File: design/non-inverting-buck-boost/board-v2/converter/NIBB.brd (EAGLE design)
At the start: 64.7 x 43.2 mm, 10 parts

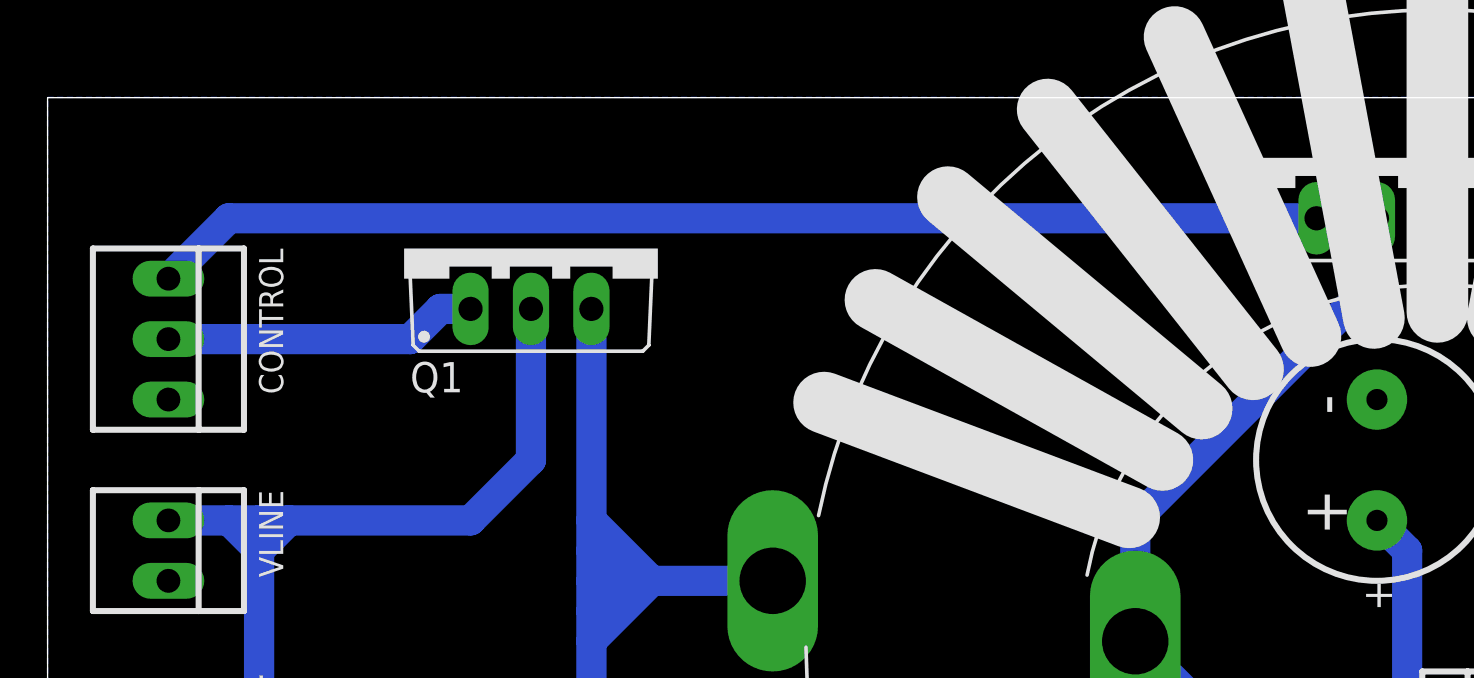
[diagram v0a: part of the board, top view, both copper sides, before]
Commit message: updated mosfet conections
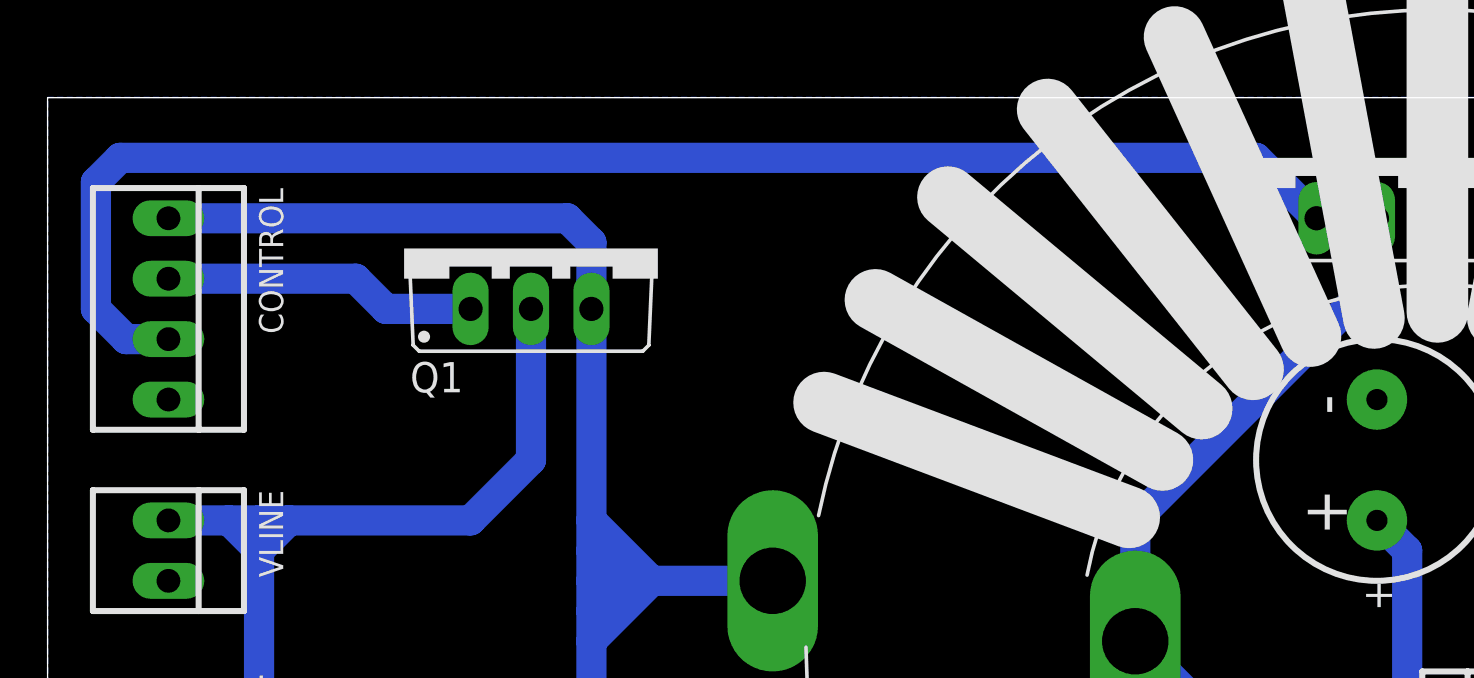
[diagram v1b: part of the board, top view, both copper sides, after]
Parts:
- CONTROL: value 22-23-2031 -> 22-23-2041; device con-molex:22-23-2031 -> con-molex:22-23-2041
- moved CONTROL 1.27 mm to (5.08, 34.3)
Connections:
- net CONTROL2 renamed N$4
- removed net CONTROL1: CONTROL.1, Q2.G
- new net N$5: CONTROL.3, Q2.G
- net GND: now also CONTROL.4; no longer CONTROL.3
- net N$1: now also CONTROL.1
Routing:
- net N$5: track 0.00 -> 61.7 mm
- net CONTROL1: track 49.3 -> 0.00 mm
- net N$1: track 42.5 -> 63.5 mm
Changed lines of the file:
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@@
 <element name="Q1" library="felippe" package="TO220BV" value="" x="20.32" y="36.83"/>
 <element name="Q2" library="felippe" package="TO220BV" value="" x="55.88" y="40.64"/>
-<element name="CONTROL" library="con-molex" package="22-23-2031" value="22-23-2031" x="5.08" y="33.02" rot="R270">
-<attribute name="MF" value="MOLEX" x="5.08" y="33.02" size="1.778" layer="27" rot="R270" display="off"/>
-<attribute name="MPN" value="22-23-2031" x="5.08" y="33.02" size="1.778" layer="27" rot="R270" display="off"/>
-<attribute name="OC_FARNELL" value="1462950" x="5.08" y="33.02" size="1.778" layer="27" rot="R270" display="off"/>
-<attribute name="OC_NEWARK" value="30C0862" x="5.08" y="33.02" size="1.778" layer="27" rot="R270" display="off"/>
-</element>
 <element name="CIN" library="capacitor" package="20ROUND40P" value="" x="8.89" y="12.7" rot="R270">
 <attribute name="DESC" value="Capacitor, polarized" x="8.89" y="12.7" size="1.778" layer="27" rot="R270" display="off"/>
+</element>
+<element name="CONTROL" library="con-molex" package="22-23-2041" value="22-23-2041" x="5.08" y="34.29" rot="R270">
+<attribute name="MF" value="MOLEX" x="5.08" y="34.29" size="1.778" layer="27" rot="R270" display="off"/>
+<attribute name="MPN" value="22-23-2041" x="5.08" y="34.29" size="1.778" layer="27" rot="R270" display="off"/>
+<attribute name="OC_FARNELL" value="1462920" x="5.08" y="34.29" size="1.778" layer="27" rot="R270" display="off"/>
+<attribute name="OC_NEWARK" value="38C0355" x="5.08" y="34.29" size="1.778" layer="27" rot="R270" display="off"/>
 </element>
 </elements>
@@
 <wire x1="20.32" y1="27.94" x2="20.32" y2="34.29" width="1.27" layer="16"/>
 </signal>
-<signal name="CONTROL1">
-<contactref element="Q2" pad="G"/>
-<contactref element="CONTROL" pad="1"/>
-<wire x1="5.08" y1="35.56" x2="7.62" y2="38.1" width="1.27" layer="16"/>
-<wire x1="7.62" y1="38.1" x2="53.34" y2="38.1" width="1.27" layer="16"/>
-</signal>
 <signal name="N$7">
 <contactref element="D2" pad="C"/>
@@
 <wire x1="22.86" y1="24.13" x2="22.86" y2="22.86" width="1.27" layer="16"/>
 <wire x1="22.86" y1="24.13" x2="22.86" y2="25.4" width="1.27" layer="16"/>
-<wire x1="22.86" y1="25.4" x2="22.86" y2="34.29" width="1.27" layer="16"/>
+<wire x1="22.86" y1="34.29" x2="22.86" y2="25.4" width="1.27" layer="16"/>
 <wire x1="22.86" y1="22.86" x2="22.86" y2="21.59" width="1.27" layer="16"/>
 <wire x1="22.86" y1="21.59" x2="22.86" y2="20.32" width="1.27" layer="16"/>
@@
 <wire x1="22.86" y1="21.59" x2="24.13" y2="22.86" width="1.27" layer="16"/>
 <wire x1="24.13" y1="22.86" x2="22.86" y2="24.13" width="1.27" layer="16"/>
+<contactref element="CONTROL" pad="1"/>
+<wire x1="5.08" y1="38.1" x2="21.844" y2="38.1" width="1.27" layer="16"/>
+<wire x1="21.844" y1="38.1" x2="22.86" y2="37.084" width="1.27" layer="16"/>
+<wire x1="22.86" y1="37.084" x2="22.86" y2="34.29" width="1.27" layer="16"/>
 </signal>
 <signal name="GND">
@@
 <contactref element="OUT" pad="2"/>
 <contactref element="Q2" pad="S"/>
-<contactref element="CONTROL" pad="3"/>
 <contactref element="CIN" pad="-"/>
-<polygon width="1.016" layer="16" spacing="0.889" pour="hatch" isolate="0.5842">
+<polygon width="1.016" layer="16" spacing="0.889" pour="hatch">
 <vertex x="0" y="43.18"/>
 <vertex x="64.77" y="43.18"/>
@@
 <vertex x="0" y="0"/>
 </polygon>
+<contactref element="CONTROL" pad="4"/>
 </signal>
-<signal name="CONTROL2">
+<signal name="N$4">
 <contactref element="CONTROL" pad="2"/>
 <contactref element="Q1" pad="G"/>
-<wire x1="5.08" y1="33.02" x2="15.24" y2="33.02" width="1.27" layer="16"/>
-<wire x1="15.24" y1="33.02" x2="16.51" y2="34.29" width="1.27" layer="16"/>
-<wire x1="16.51" y1="34.29" x2="17.78" y2="34.29" width="1.27" layer="16"/>
+<wire x1="5.08" y1="35.56" x2="12.954" y2="35.56" width="1.27" layer="16"/>
+<wire x1="12.954" y1="35.56" x2="14.224" y2="34.29" width="1.27" layer="16"/>
+<wire x1="14.224" y1="34.29" x2="17.78" y2="34.29" width="1.27" layer="16"/>
+</signal>
+<signal name="N$5">
+<contactref element="CONTROL" pad="3"/>
+<contactref element="Q2" pad="G"/>
+<wire x1="5.08" y1="33.02" x2="3.302" y2="33.02" width="1.27" layer="16"/>
+<wire x1="3.302" y1="33.02" x2="2.032" y2="34.29" width="1.27" layer="16"/>
+<wire x1="2.032" y1="34.29" x2="2.032" y2="39.624" width="1.27" layer="16"/>
+<wire x1="2.032" y1="39.624" x2="3.048" y2="40.64" width="1.27" layer="16"/>
+<wire x1="3.048" y1="40.64" x2="50.8" y2="40.64" width="1.27" layer="16"/>
+<wire x1="50.8" y1="40.64" x2="53.34" y2="38.1" width="1.27" layer="16"/>
 </signal>
 </signals>

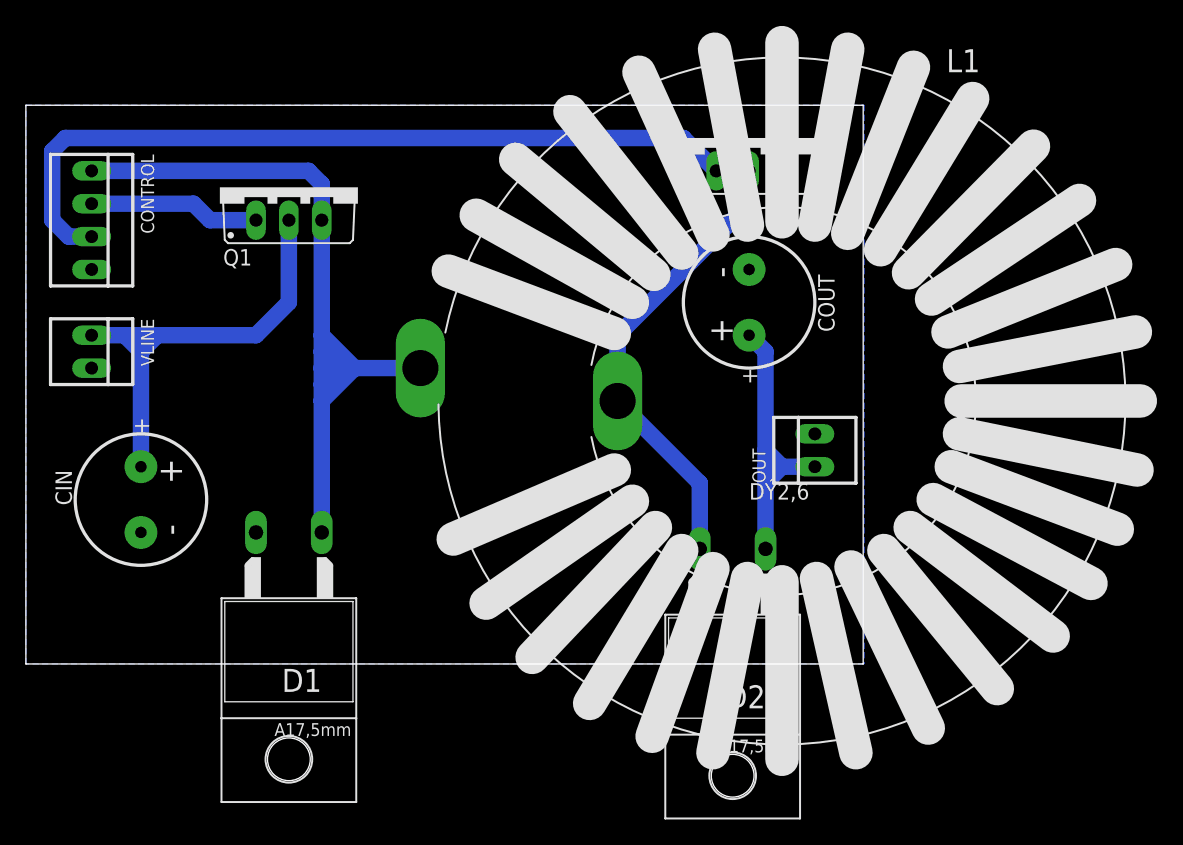
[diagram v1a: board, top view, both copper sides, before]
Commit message: added drill holes
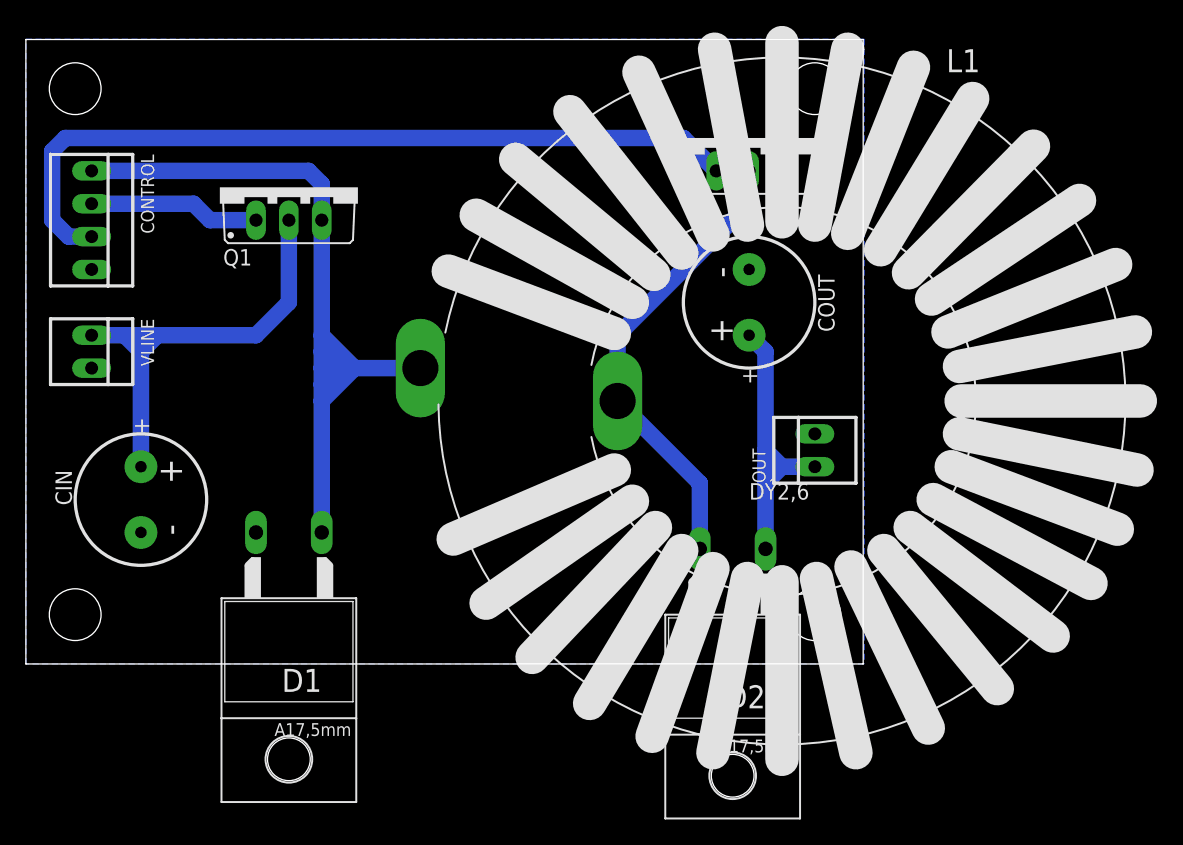
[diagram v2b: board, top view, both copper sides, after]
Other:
- board size 64.7 x 43.2 mm -> 64.7 x 48.2 mm
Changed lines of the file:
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@@
 <setting verticaltext="up"/>
 </settings>
-<grid distance="10" unitdist="mil" unit="mil" style="lines" multiple="1" display="yes" altdistance="0.025" altunitdist="inch" altunit="inch"/>
+<grid distance="50" unitdist="mil" unit="mil" style="lines" multiple="1" display="yes" altdistance="0.025" altunitdist="inch" altunit="inch"/>
 <layers>
 <layer number="1" name="Top" color="4" fill="1" visible="yes" active="yes"/>
@@
 <plain>
 <wire x1="0" y1="0" x2="64.694" y2="0" width="0" layer="20"/>
-<wire x1="64.694" y1="0" x2="64.694" y2="43.17" width="0" layer="20"/>
-<wire x1="64.694" y1="43.17" x2="0" y2="43.17" width="0" layer="20"/>
-<wire x1="0" y1="43.17" x2="0" y2="0" width="0" layer="20"/>
+<wire x1="64.694" y1="0" x2="64.694" y2="48.25" width="0" layer="20"/>
+<wire x1="64.694" y1="48.25" x2="0" y2="48.25" width="0" layer="20"/>
+<wire x1="0" y1="48.25" x2="0" y2="0" width="0" layer="20"/>
+<hole x="3.81" y="44.45" drill="4"/>
+<hole x="60.96" y="44.45" drill="4"/>
+<hole x="3.81" y="3.81" drill="4"/>
+<hole x="60.96" y="3.81" drill="4"/>
 </plain>
 <attributes>
@@
 <contactref element="CIN" pad="-"/>
 <polygon width="1.016" layer="16" spacing="0.889" pour="hatch">
-<vertex x="0" y="43.18"/>
-<vertex x="64.77" y="43.18"/>
+<vertex x="0" y="48.26"/>
+<vertex x="64.77" y="48.26"/>
 <vertex x="64.77" y="0"/>
 <vertex x="0" y="0"/>
